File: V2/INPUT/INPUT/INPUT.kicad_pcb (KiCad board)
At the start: 2 copper layers, 100 x 30 mm, 54 parts, among them J1 Conn_01x03, J2 USB_C_Receptacle_USB2.0_16P, J3 Conn_01x03, J4 Conn_01x03, J5 Conn_01x03, J6 Conn_01x03, J7 Conn_01x03, J8 Conn_01x03, J9 Conn_01x03, Q1 QM6006D, Q2 QM6006D, Q3 QM6006D, Q4 QM6006D, Q5 QM6006D, Q6 QM6006D, Q7 QM6006D, Q8 QM6006D, SW1 SW_SPST, SW2 SW_SPST, SW3 SW_SPST, SW4 SW_SPST, SW5 SW_SPST, SW6 SW_SPST, SW7 SW_SPST, SW8 SW_SPST, U1 USBLC6-2P6

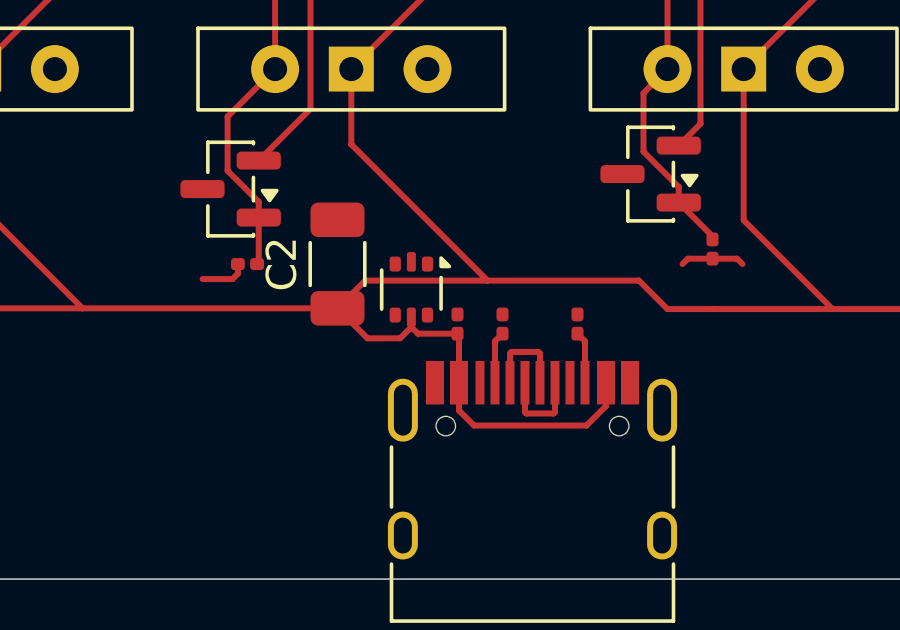
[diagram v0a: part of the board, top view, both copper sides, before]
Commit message: Auto-update: 15.04.2026 12:38:29,38
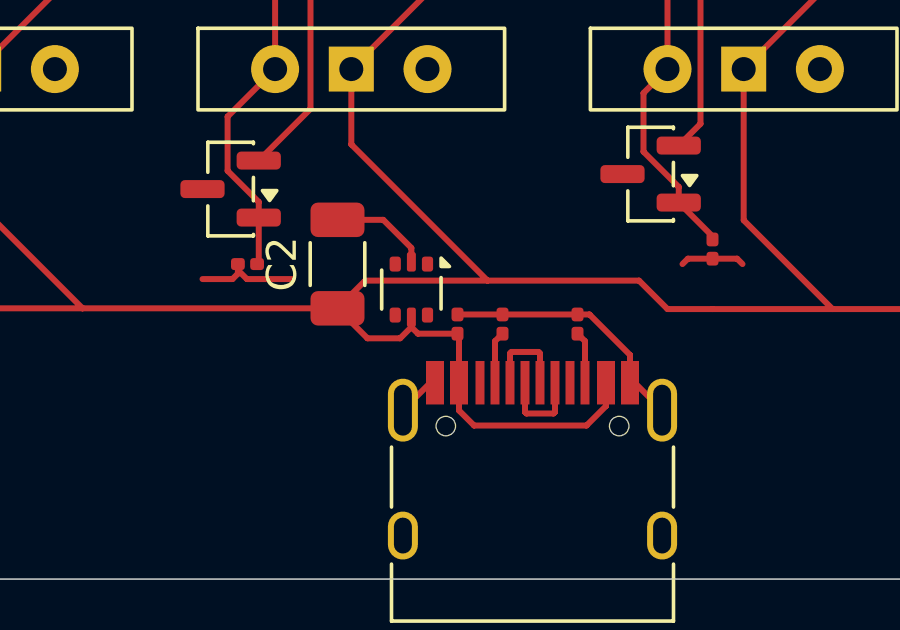
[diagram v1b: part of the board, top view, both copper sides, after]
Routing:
- net GND: track 17.8 -> 33.4 mm
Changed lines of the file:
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@@
+	)
+	(segment
+		(start 49 21.18)
+		(end 51.5 21.18)
+		(width 0.2)
+		(layer "F.Cu")
+		(net 2)
 	)
 	(segment
@@
 	)
 	(segment
+		(start 53.25 22.53)
+		(end 53.25 23.455)
+		(width 0.2)
+		(layer "F.Cu")
+		(net 2)
+	)
+	(segment
 		(start 90.82 19.32)
 		(end 90.5 19)
@@
 	)
 	(segment
+		(start 40.480001 20)
+		(end 42 20)
+		(width 0.2)
+		(layer "F.Cu")
+		(net 2)
+	)
+	(segment
 		(start 40.18 19.82)
 		(end 40 20)
@@
 	)
 	(segment
+		(start 40.18 19.5)
+		(end 40.18 19.699999)
+		(width 0.2)
+		(layer "F.Cu")
+		(net 2)
+	)
+	(segment
+		(start 45.025 18.025)
+		(end 43.5 18.025)
+		(width 0.2)
+		(layer "F.Cu")
+		(net 2)
+	)
+	(segment
 		(start 69.32 19.32)
 		(end 69.5 19.5)
@@
 	)
 	(segment
+		(start 53.25 23.455)
+		(end 53.405 23.455)
+		(width 0.2)
+		(layer "F.Cu")
+		(net 2)
+	)
+	(segment
 		(start 7.32 19.32)
 		(end 7.5 19.5)
@@
 	)
 	(segment
+		(start 53.405 23.455)
+		(end 54.32 24.37)
+		(width 0.2)
+		(layer "F.Cu")
+		(net 2)
+	)
+	(segment
+		(start 51.9 21.18)
+		(end 53.25 22.53)
+		(width 0.2)
+		(layer "F.Cu")
+		(net 2)
+	)
+	(segment
 		(start 79.18 19.32)
 		(end 79 19.5)
@@
 	)
 	(segment
+		(start 47.5 21.18)
+		(end 49 21.18)
+		(width 0.2)
+		(layer "F.Cu")
+		(net 2)
+	)
+	(segment
 		(start 56.82 19.32)
 		(end 56 19.32)
@@
 	)
 	(segment
+		(start 45.9625 19.425)
+		(end 45.9625 18.9625)
+		(width 0.2)
+		(layer "F.Cu")
+		(net 2)
+	)
+	(segment
+		(start 46.595 23.455)
+		(end 45.68 24.37)
+		(width 0.2)
+		(layer "F.Cu")
+		(net 2)
+	)
+	(segment
+		(start 51.5 21.18)
+		(end 51.9 21.18)
+		(width 0.2)
+		(layer "F.Cu")
+		(net 2)
+	)
+	(segment
 		(start 31.82 19.32)
 		(end 32 19.5)
@@
 	)
 	(segment
+		(start 45.9625 18.9625)
+		(end 45.025 18.025)
+		(width 0.2)
+		(layer "F.Cu")
+		(net 2)
+	)
+	(segment
 		(start 55.18 19.32)
 		(end 56 19.32)
@@
 	)
 	(segment
+		(start 40.18 19.699999)
+		(end 40.480001 20)
+		(width 0.2)
+		(layer "F.Cu")
+		(net 2)
+	)
+	(segment
 		(start 18.5 19.32)
 		(end 19.32 19.32)
@@
 		(width 0.2)
 		(layer "F.Cu")
+		(net 2)
+	)
+	(segment
+		(start 46.75 23.455)
+		(end 46.595 23.455)
+		(width 0.2)
+		(layer "F.Cu")
